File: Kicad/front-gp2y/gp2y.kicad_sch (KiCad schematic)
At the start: 14 parts, among them IC1 MCP1755-50, K1 GP2Y, K2 MCU

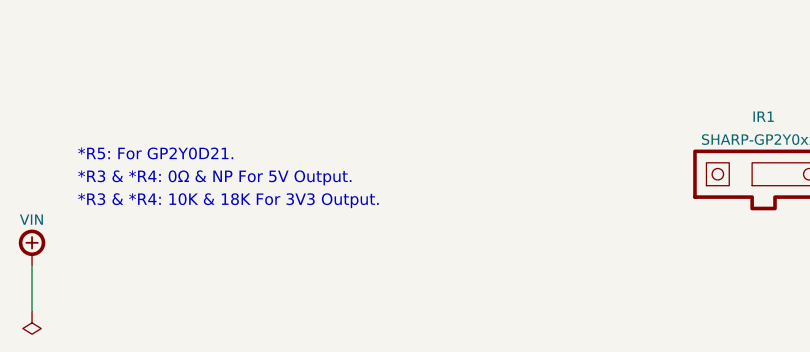
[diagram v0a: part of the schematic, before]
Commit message: Draft
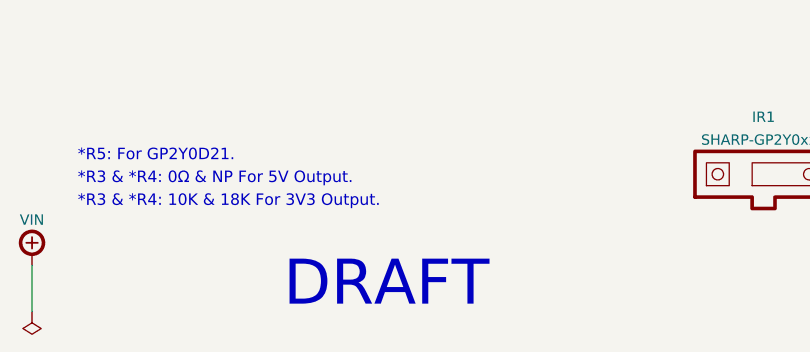
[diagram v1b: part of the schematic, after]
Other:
- note added: "DRAFT"
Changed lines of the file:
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@@
     (effects (font (size 1.27 1.27)) (justify left bottom))
+  )
+  (text "DRAFT" (at 208.28 190.5 0)
+    (effects (font (size 5 5)) (justify left bottom))
   )
   (text "*" (at 147.32 86.36 0)

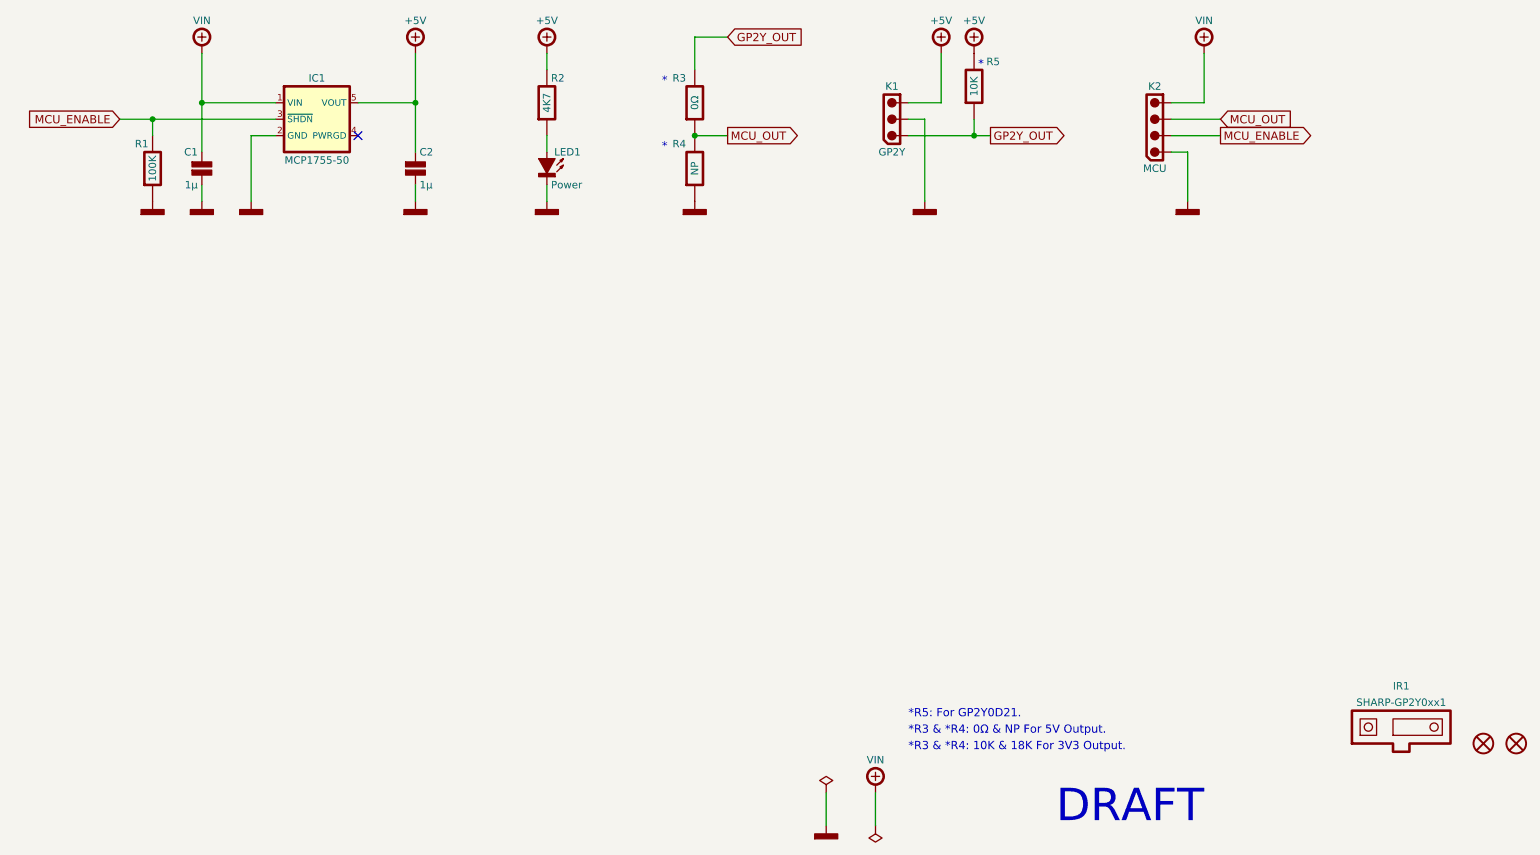
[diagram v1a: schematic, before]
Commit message: Update GP2Y
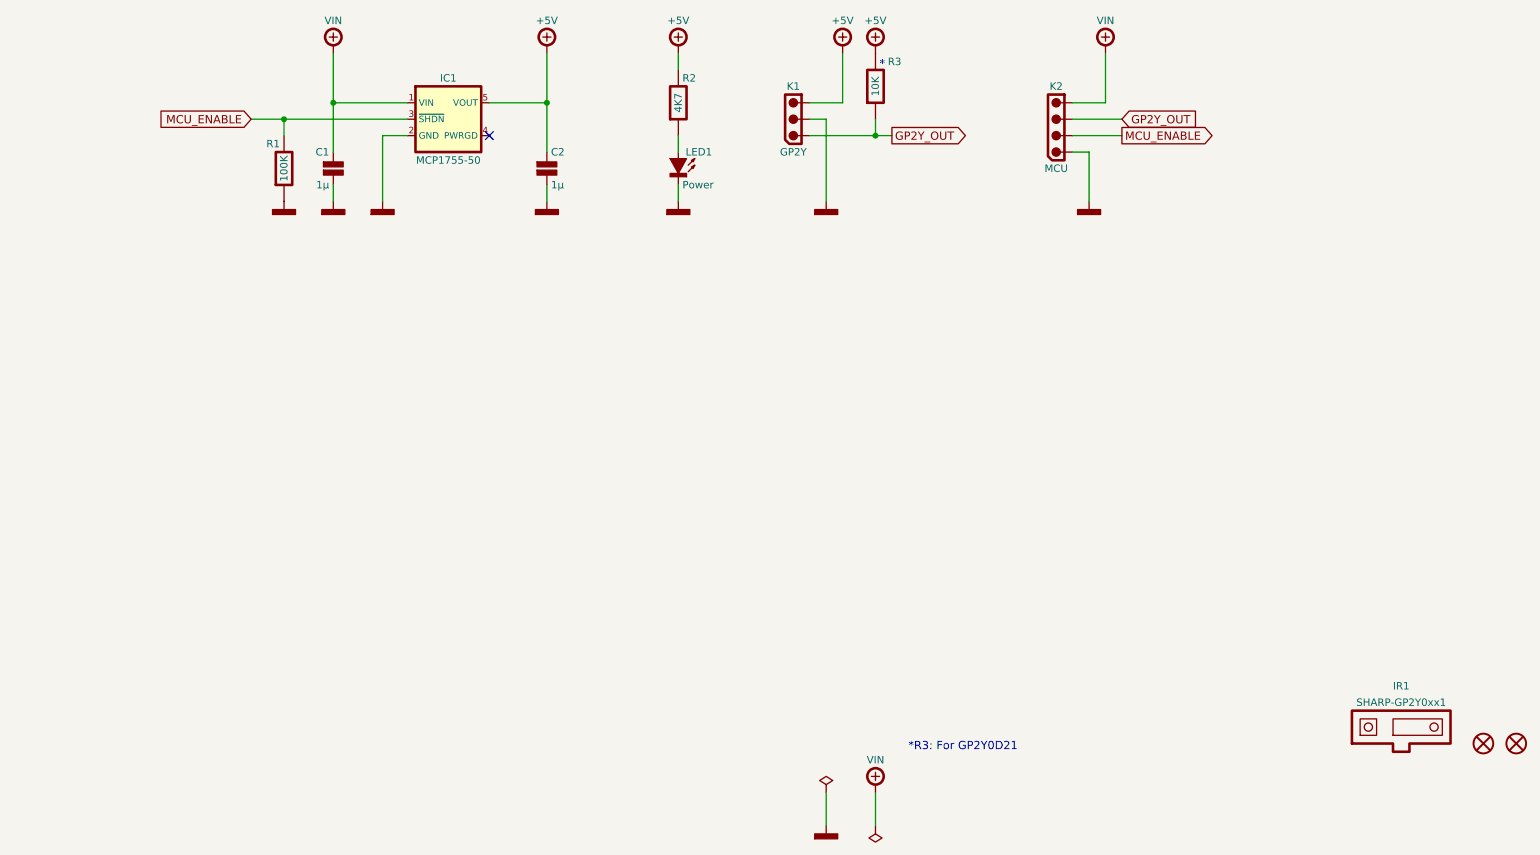
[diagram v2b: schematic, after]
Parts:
- removed R3: 0Ω, tronixio:RESISTOR-1206, symbol tronixio:R-1206
- removed R4: NP, tronixio:RESISTOR-1206, symbol tronixio:R-1206
- renumbered R5 to R3
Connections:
- net MCU_OUT is gone; now on net GP2Y_OUT: K2.3
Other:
- note added: "*R3: For GP2Y0D21"
- note removed: "*R3 & *R4: 0Ω & NP For 5V Output."
- note removed: "*R3 & *R4: 10K & 18K For 3V3 Output."
- note removed: "*R5: For GP2Y0D21."
- note removed: "DRAFT"
- moved on the sheet: C1, C2, IC1, K1, K2, LED1, R1, R2, R3

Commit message: Update gp2y.kicad_sch
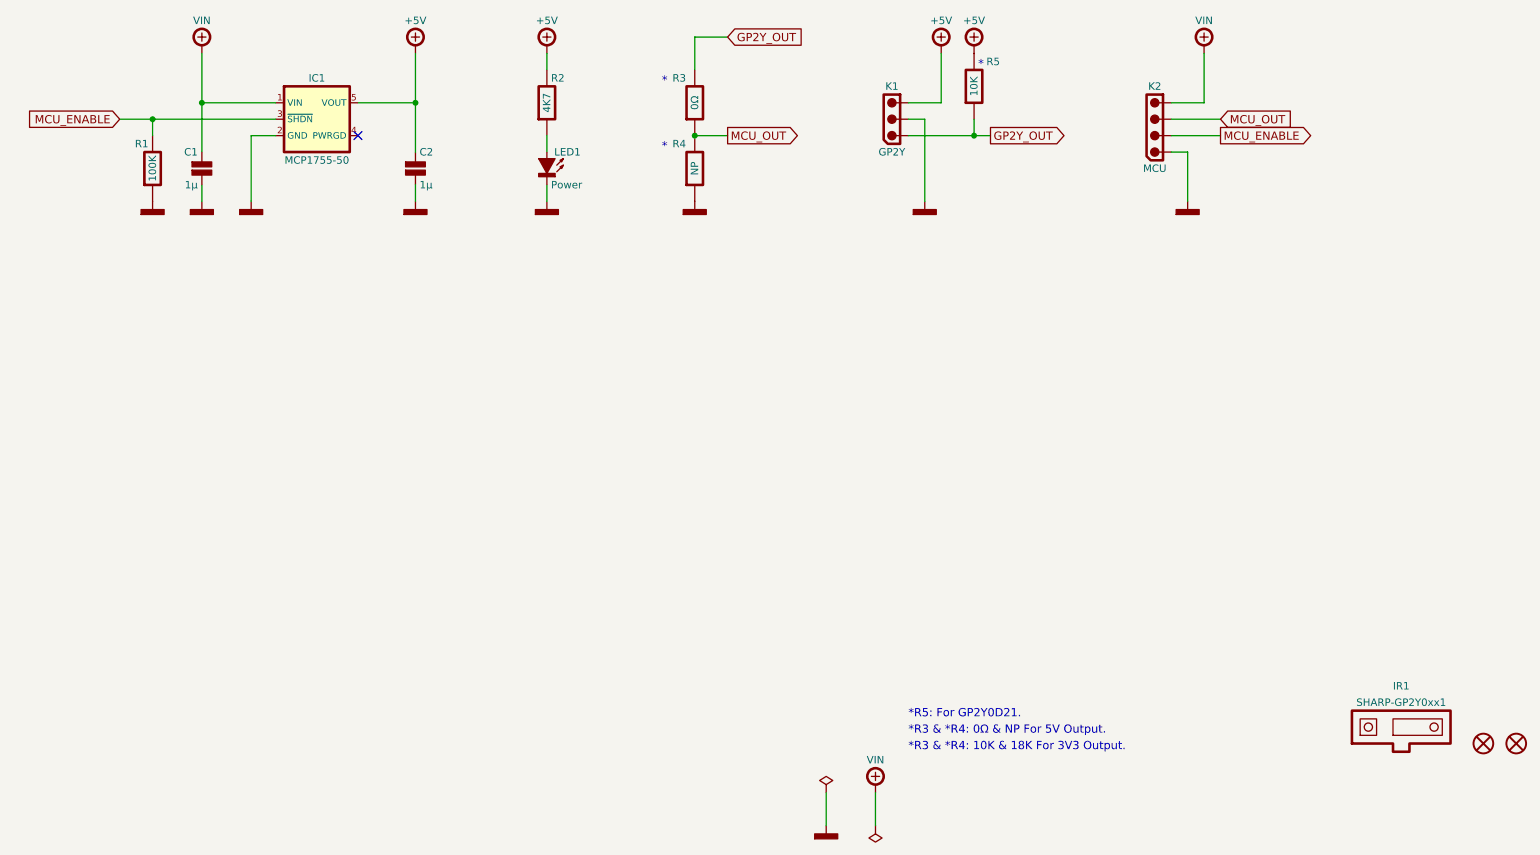
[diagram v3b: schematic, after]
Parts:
- added R3: 0Ω, tronixio:RESISTOR-1206, symbol tronixio:R-1206
- added R4: NP, tronixio:RESISTOR-1206, symbol tronixio:R-1206
- renumbered R3 to R5
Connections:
- net GND: now also R4.2
- net GP2Y_OUT: now also R3.1; no longer K2.3
- new net MCU_OUT: K2.3, R3.2, R4.1
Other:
- note added: "*R3 & *R4: 0Ω & NP For 5V Output."
- note added: "*R3 & *R4: 10K & 18K For 3V3 Output."
- note added: "*R5: For GP2Y0D21."
- note removed: "*R3: For GP2Y0D21"
- moved on the sheet: C1, C2, IC1, K1, K2, LED1, R1, R2, R5
